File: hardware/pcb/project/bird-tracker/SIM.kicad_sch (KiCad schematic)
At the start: 1 part, among them U3 SIM7080G

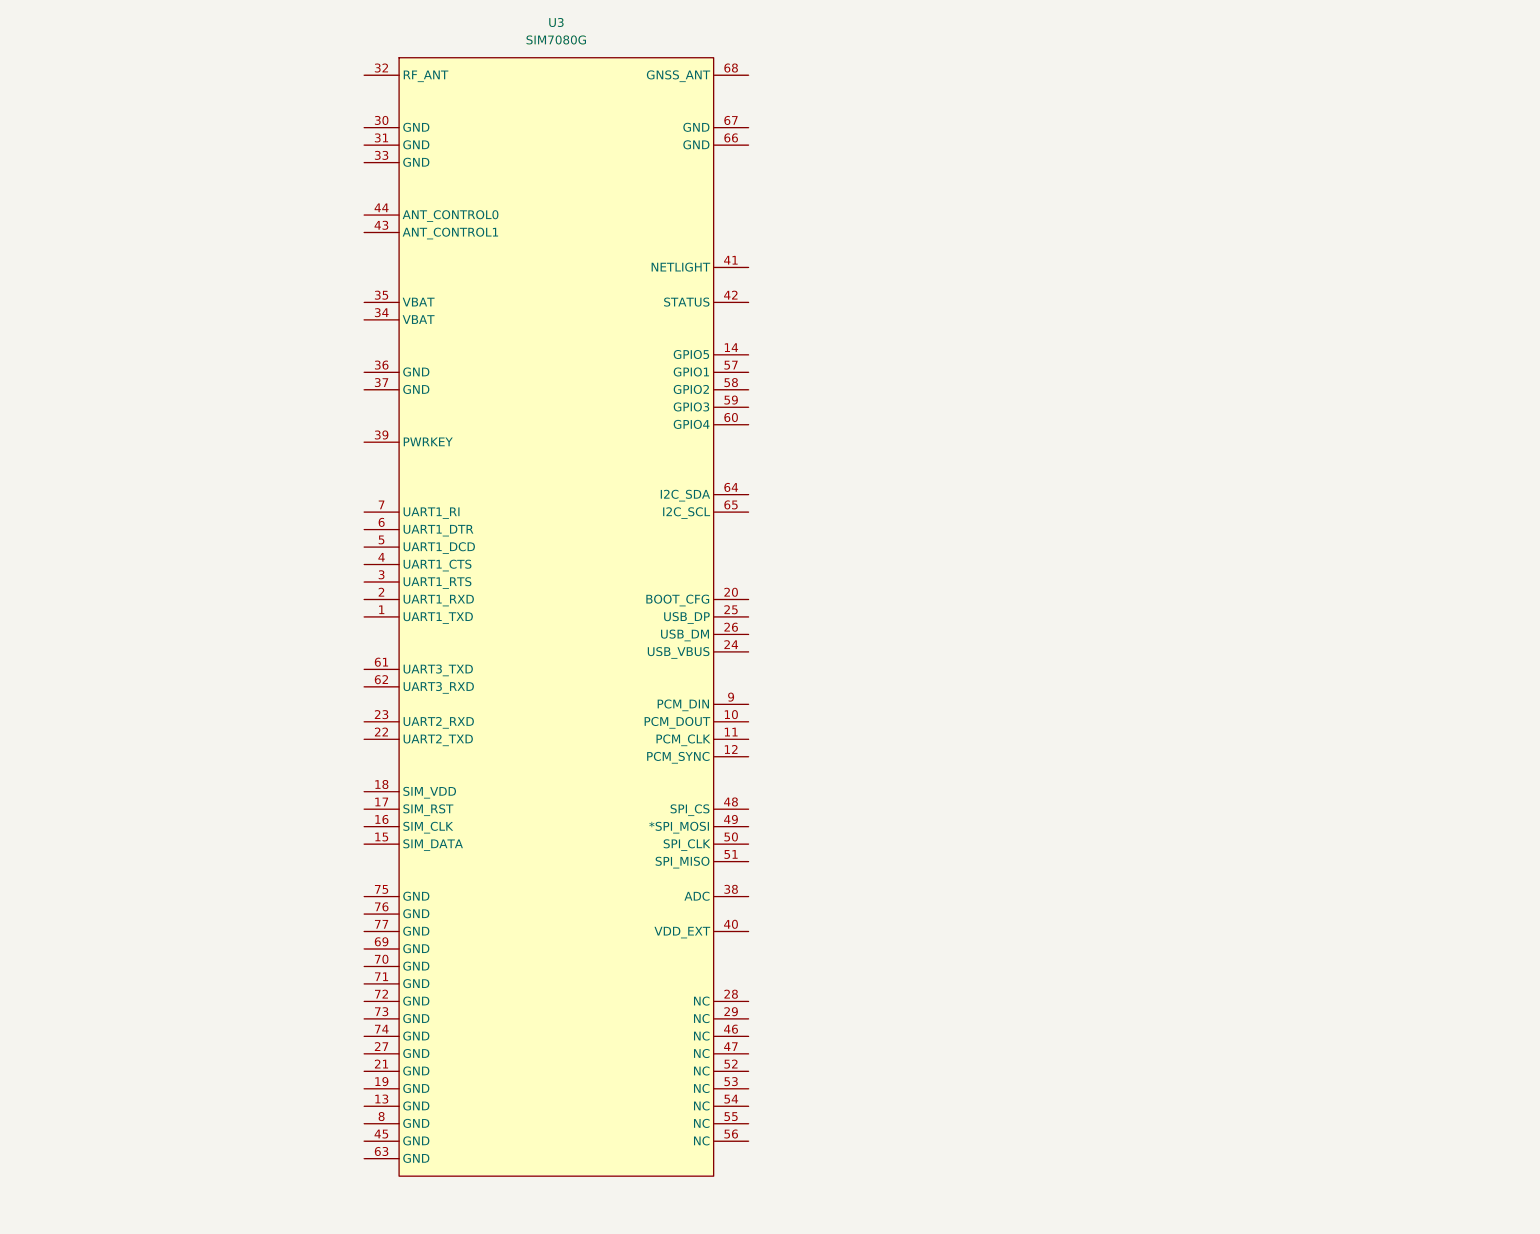
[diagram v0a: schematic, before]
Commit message: SIM sheet complete
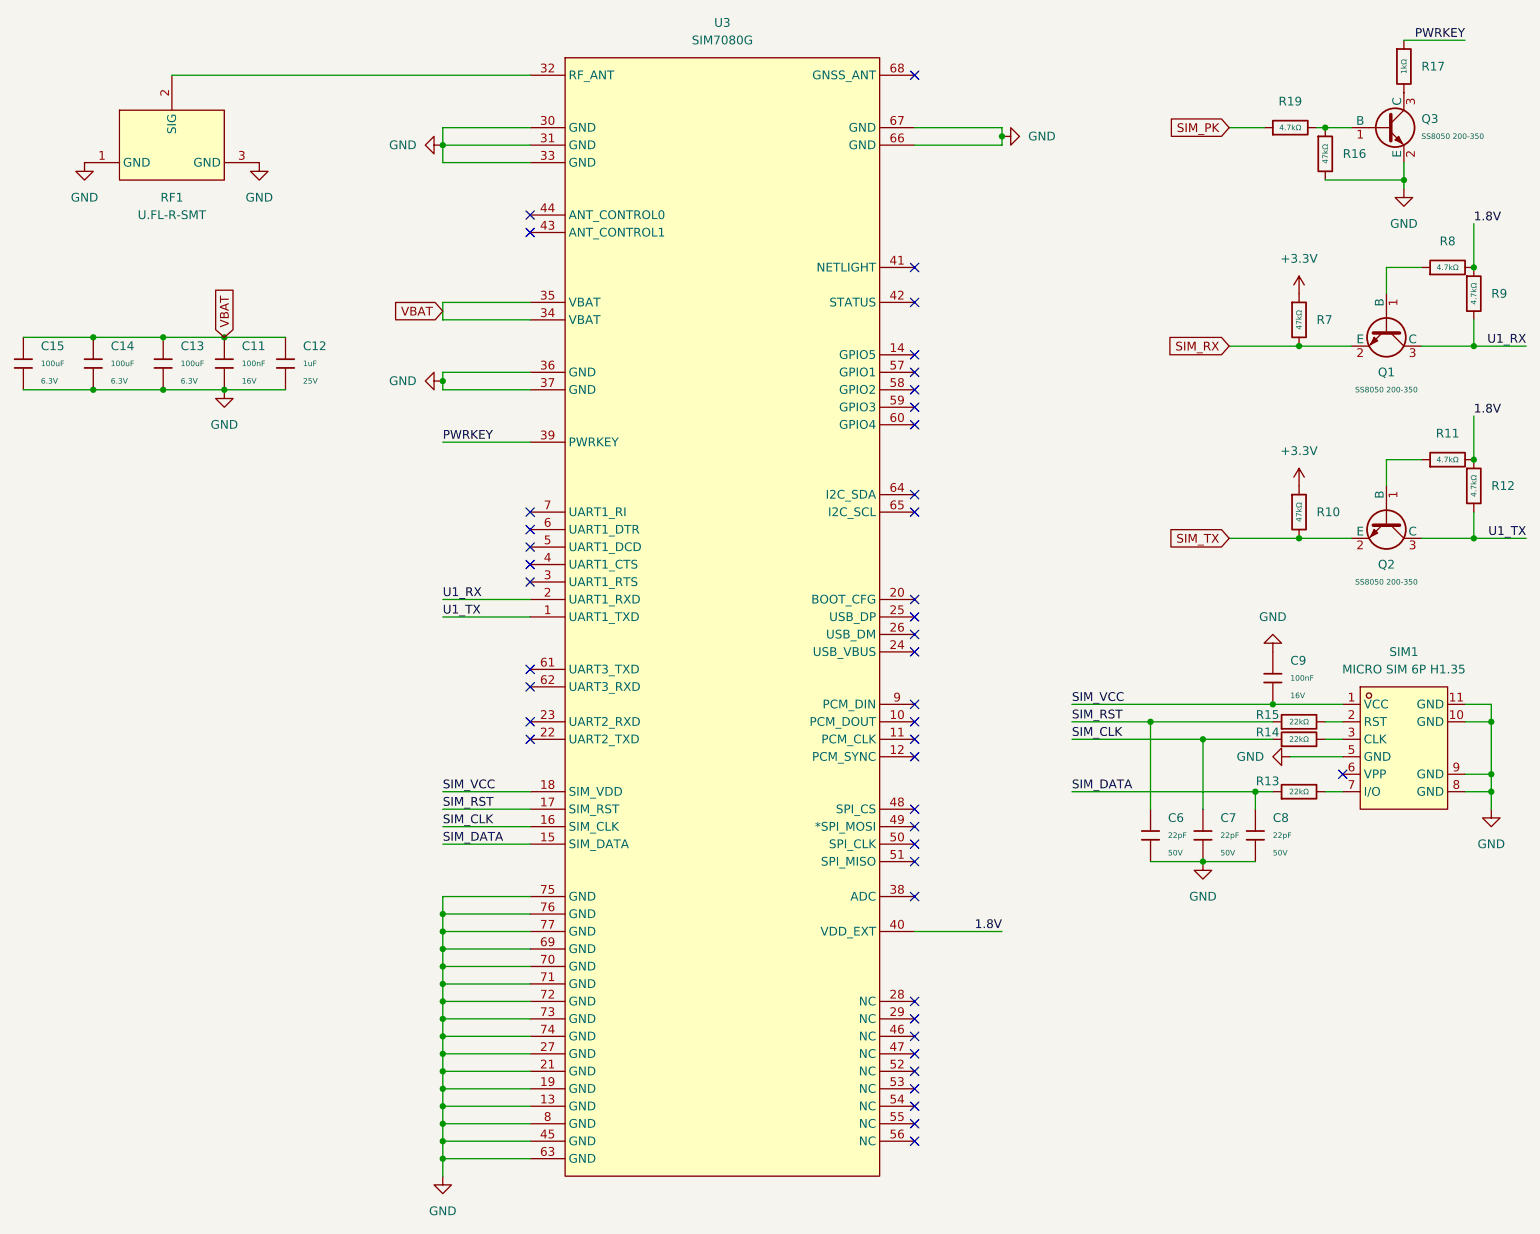
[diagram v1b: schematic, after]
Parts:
- added C11, C9: 100nF, PCM_JLCPCB:C_0402, symbol PCM_JLCPCB-Capacitors:0402,100nF
- added C12: 1uF, PCM_JLCPCB:C_0402, symbol PCM_JLCPCB-Capacitors:0402,1uF
- added C13, C14, C15: 100uF, PCM_JLCPCB:C_1206, symbol PCM_JLCPCB-Capacitors:1206,100uF
- added C6, C7, C8: 22pF, PCM_JLCPCB:C_0402, symbol PCM_JLCPCB-Capacitors:0402,22pF
- added Q1, Q2, Q3: SS8050 200-350, PCM_JLCPCB:Q_SOT-23, symbol PCM_JLCPCB-Transistors:NPN,SS8050 200-350
- added R10, R16, R7: 47kΩ, PCM_JLCPCB:R_0402, symbol PCM_JLCPCB-Resistors:0402,47kΩ
- added R11, R12, R19, R8, R9: 4.7kΩ, PCM_JLCPCB:R_0402, symbol PCM_JLCPCB-Resistors:0402,4.7kΩ
- added R13, R14, R15: 22kΩ, PCM_JLCPCB:R_0402, symbol PCM_JLCPCB-Resistors:0402,22kΩ
- added R17: 1kΩ, PCM_JLCPCB:R_0402, symbol PCM_JLCPCB-Resistors:0402,1kΩ
- added RF1: U.FL-R-SMT, bird-tracker:ANT-SMD_U.FL-R-SMT10, symbol bird-tracker:U.FL-R-SMT
- added SIM1: MICRO SIM 6P H1.35, bird-tracker:SIM-SMD_MICRO-SIM-6P-H1.35, symbol bird-tracker:MICROSIM6PH1.35
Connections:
- net U1_TX: now reaches U3.1 (UART1_TXD)
- net U1_TX: now also Q2.3 (C), R12.2
- net GND: now reaches U3.13 (GND)
- net GND: now also U3.19 (GND), U3.21 (GND), U3.27 (GND), U3.30 (GND), U3.31 (GND), U3.33 (GND), U3.36 (GND), U3.37 (GND), U3.45 (GND), U3.63 (GND), U3.66 (GND), U3.67 (GND), U3.69 (GND), U3.70 (GND), U3.71 (GND), U3.72 (GND), U3.73 (GND), U3.74 (GND), U3.75 (GND), U3.76 (GND), U3.77 (GND), U3.8 (GND), C11.2, C12.2, C13.2, C14.2, C15.2, C6.2, C7.2, C8.2, C9.1, Q3.2 (E), R16.2, RF1.1 (GND), RF1.3 (GND), SIM1.10 (GND), SIM1.11 (GND), SIM1.5 (GND), SIM1.8 (GND), SIM1.9 (GND)
- net SIM_DATA: now reaches U3.15 (SIM_DATA)
- net SIM_DATA: now also C8.1, R13.1
- net SIM_CLK: now reaches U3.16 (SIM_CLK)
- net SIM_CLK: now also C7.1, R14.1
- net SIM_RST: now reaches U3.17 (SIM_RST)
- net SIM_RST: now also C6.1, R15.1
- net SIM_VCC: now reaches U3.18 (SIM_VDD)
- net SIM_VCC: now also C9.2, SIM1.1 (VCC)
- net U1_RX: now reaches U3.2 (UART1_RXD)
- net U1_RX: now also Q1.3 (C), R9.2
- net at U3.32 (RF_ANT): now also RF1.2 (SIG)
- net VBAT: now reaches U3.34 (VBAT)
- net VBAT: now also U3.35 (VBAT), C11.1, C12.1, C13.1, C14.1, C15.1
- net PWRKEY: now reaches U3.39 (PWRKEY)
- net PWRKEY: now also R17.1
- net 1.8V: now reaches U3.40 (VDD_EXT)
- net 1.8V: now also R11.2, R12.1, R8.2, R9.1
- new net: R15.2, SIM1.2 (RST)
- new net: R14.2, SIM1.3 (CLK)
- new net: R13.2, SIM1.7 (I/O)
- new net: Q1.1 (B), R8.1
- new net: Q2.1 (B), R11.1
- new net: Q3.1 (B), R16.1, R19.2
- new net: Q3.3 (C), R17.2
- new net +3.3V: R10.1, R7.1
- new net SIM_PK: R19.1
- new net SIM_RX: Q1.2 (E), R7.2
- new net SIM_TX: Q2.2 (E), R10.2
- no-connect marks 0 -> 44
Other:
- title: (none) -> Bird Tracker - SIM
- moved on the sheet: U3
